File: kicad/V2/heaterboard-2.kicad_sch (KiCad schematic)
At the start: 10 parts, among them J1 Screw_Terminal_01x02, J2 Conn_01x05_Pin, Q1 Q_NMOS_GDS, U1 LM317_TO-220, U2 LM7805_TO220

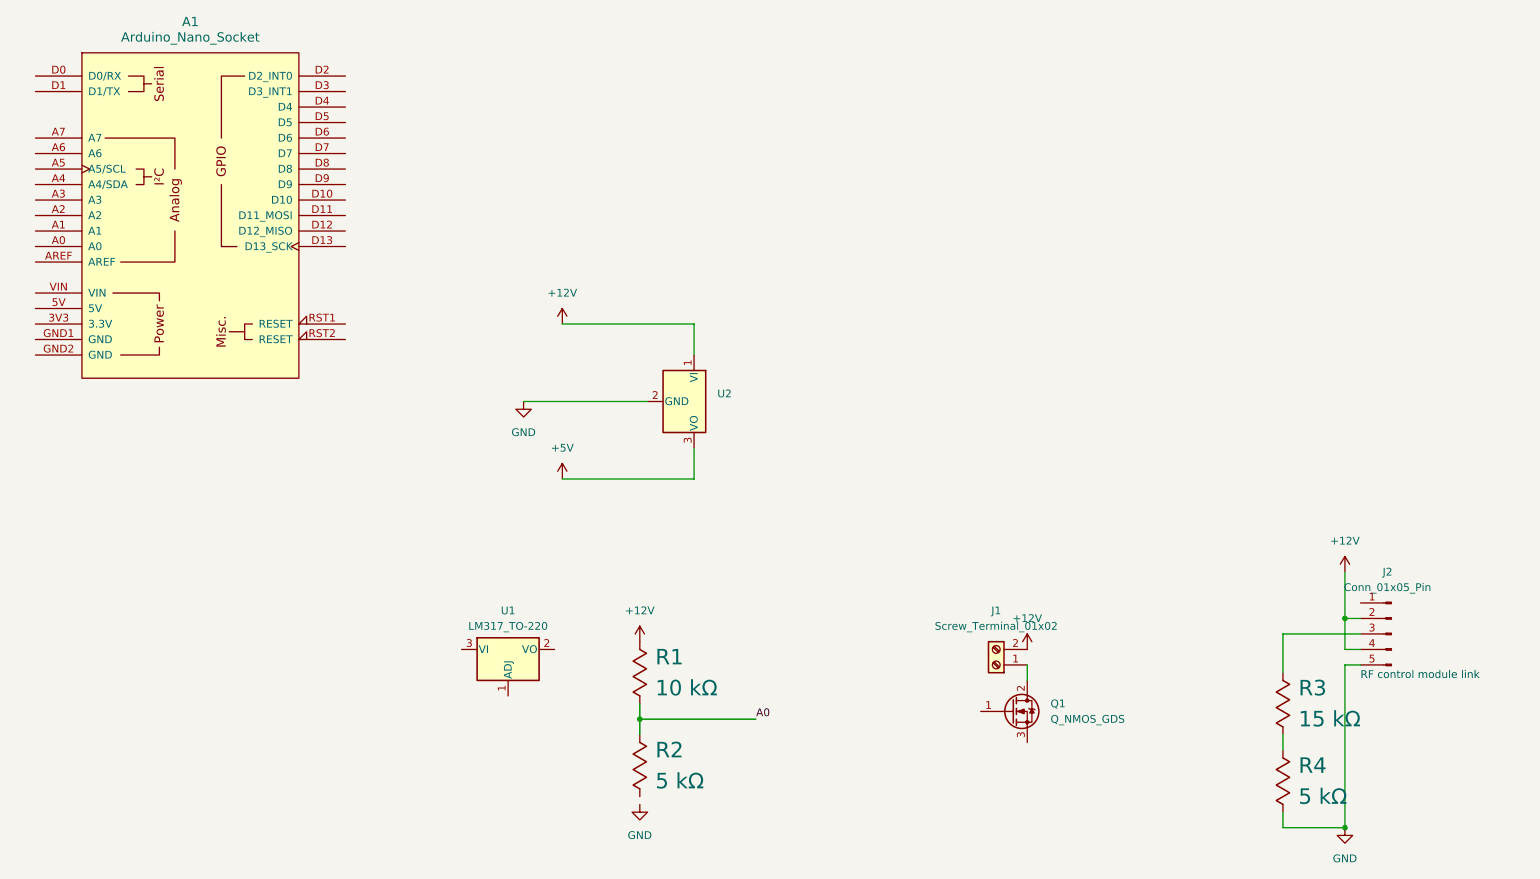
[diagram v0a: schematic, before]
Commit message: End of class 1 feb
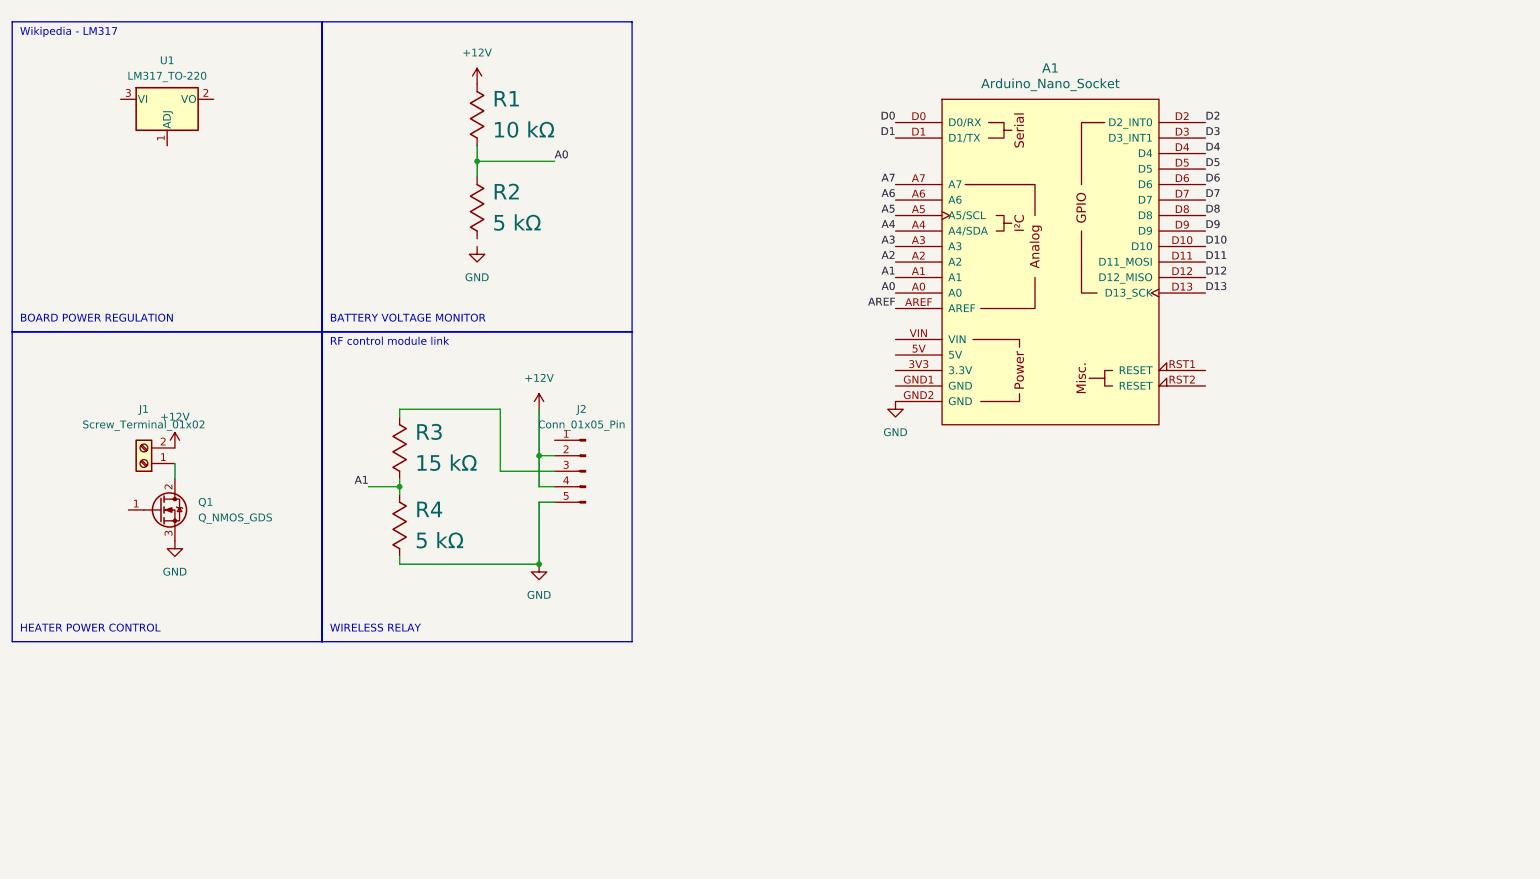
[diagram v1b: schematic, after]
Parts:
- removed U2: LM7805_TO220, Package_TO_SOT_THT:TO-220-3_Vertical, symbol Regulator_Linear:LM7805_TO220
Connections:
- net A0: now also A1.A0
- net GND: now also A1.GND2 (GND), Q1.3 (S)
- net A1: now reaches A1.A1
- net A1: now also R3.2 (-), R4.1 (+)
- net A2: now reaches A1.A2
- net A3: now reaches A1.A3
- net A4: now reaches A1.A4 (A4/SDA)
- net A5: now reaches A1.A5 (A5/SCL)
- net A6: now reaches A1.A6
- net A7: now reaches A1.A7
- net AREF: now reaches A1.AREF
- net D0: now reaches A1.D0 (D0/RX)
- net D1: now reaches A1.D1 (D1/TX)
- net D10: now reaches A1.D10
- net D11: now reaches A1.D11 (D11_MOSI)
- net D12: now reaches A1.D12 (D12_MISO)
- net D13: now reaches A1.D13 (D13_SCK)
- net D2: now reaches A1.D2 (D2_INT0)
- net D3: now reaches A1.D3 (D3_INT1)
- net D4: now reaches A1.D4
- net D5: now reaches A1.D5
- net D6: now reaches A1.D6
- net D7: now reaches A1.D7
- net D8: now reaches A1.D8
- net D9: now reaches A1.D9
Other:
- note added: "BATTERY VOLTAGE MONITOR"
- note added: "BOARD POWER REGULATION"
- note added: "HEATER POWER CONTROL"
- note added: "WIRELESS RELAY"
- note added: "Wikipedia - LM317"
- company: (none) -> ME692
- title: (none) -> Windshield Heater
- moved on the sheet: A1, J1, J2, Q1, R1, R2, R3, R4, U1
